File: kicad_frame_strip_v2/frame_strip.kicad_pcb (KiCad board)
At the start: 2 copper layers, 42.5 x 58.5 mm, 61 parts, among them J1 PROGRAM, J10 HEADER_1, J11 HEADER_1, J12 HEADER_1, J2 USART2, J3 HEADER_4, J4 HEADER_4, J5 HEADER_4, J6 HEADER_2, J7 DC_POWER_JACK, J8 SPI1, J9 HEADER_1, Q1 MOS_N_GDS, Q2 MOS_N_GDS, Q3 MOS_N_GDS, Q4 MOS_N_GDS, Q5 MOS_N_GDS, Q6 MOS_N_GDS, Q7 MOS_N_GDS, Q8 MOS_N_GDS, Q9 MOS_N_GDS, SW1 SW_PUSH, SW2 SW_PUSH, SW3 SW_SPDT, U1 STM32F100_LQFP48, U6 sot223

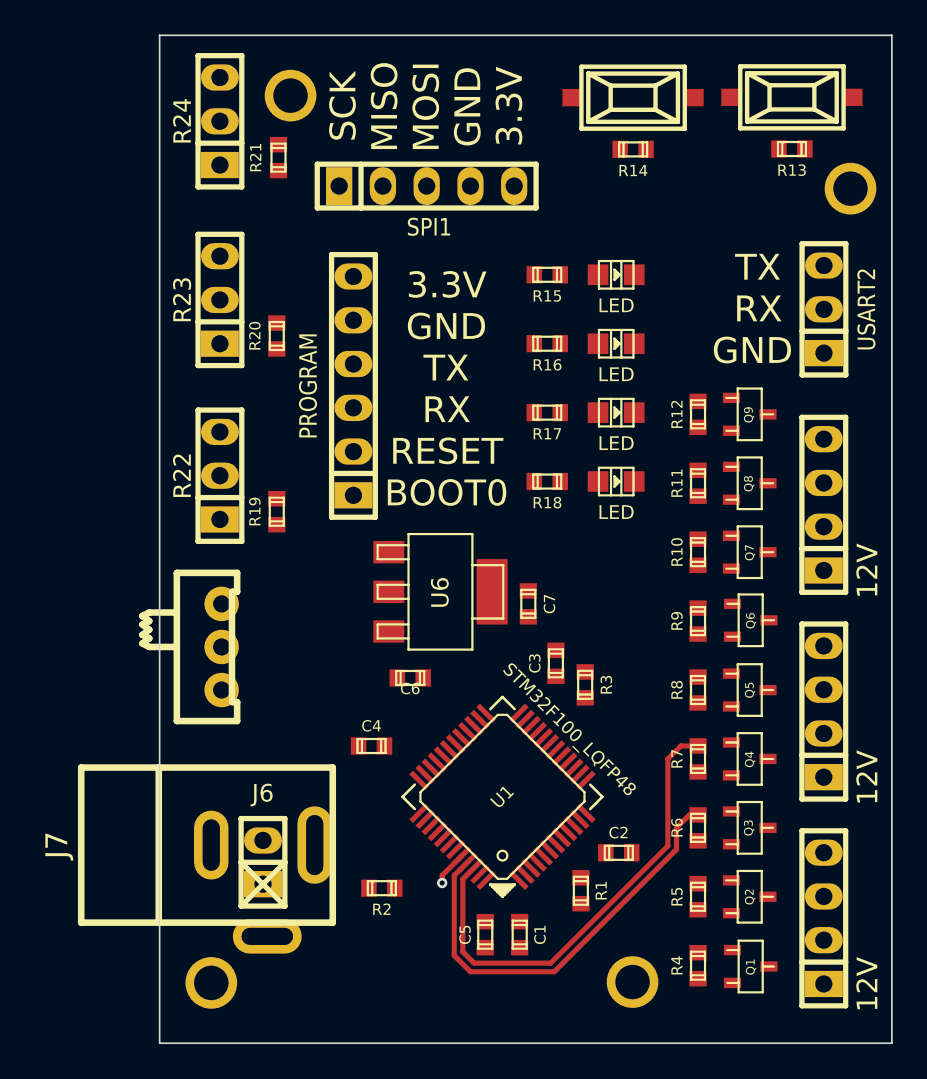
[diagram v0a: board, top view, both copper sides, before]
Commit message: PCB, code
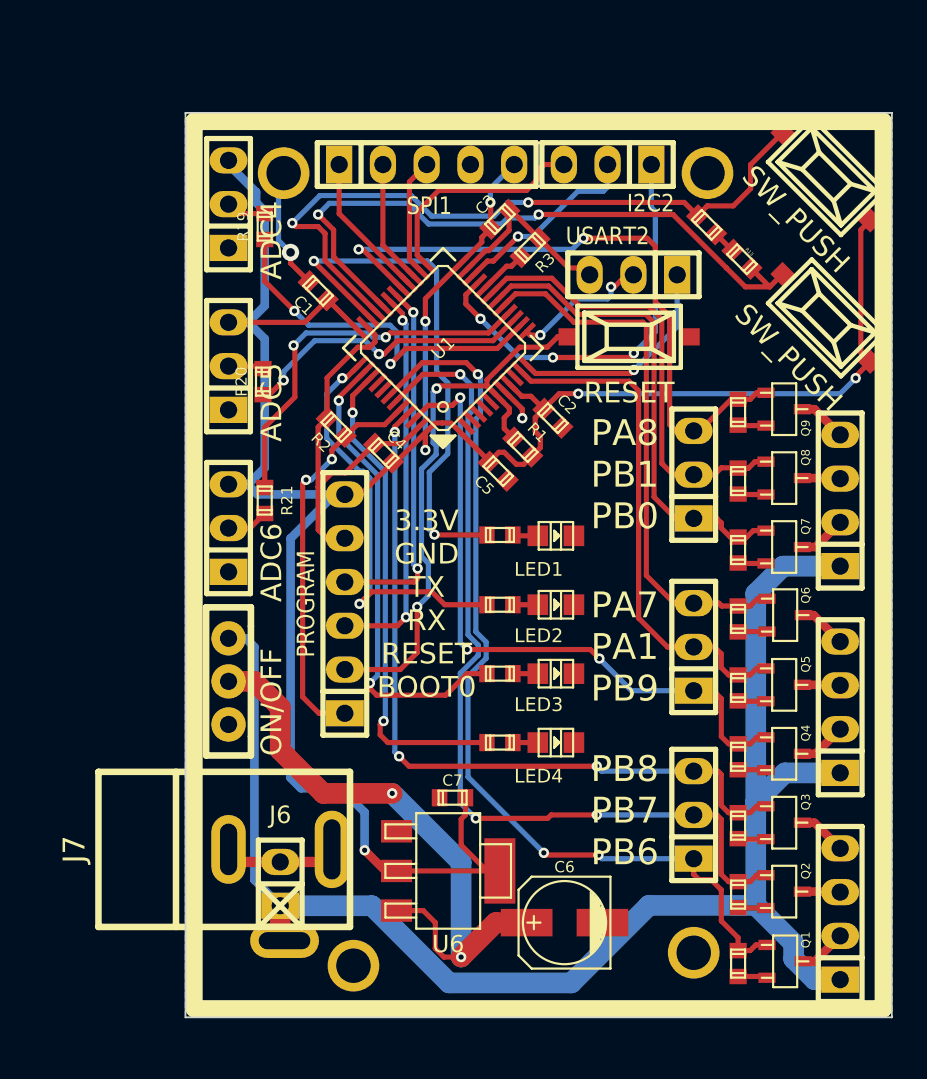
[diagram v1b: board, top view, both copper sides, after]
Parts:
- removed R22, R23: POT, w_pin_strip:pin_socket_3
- added ADC5: POT, w_pin_strip:pin_socket_3, F.Cu at (131.0, 98.2)
- added ADC6: POT, w_pin_strip:pin_socket_3, F.Cu at (131.0, 107.6)
- added J13: HEADER_3, w_pin_strip:pin_socket_3, F.Cu at (158.0, 124.2)
- added J14: HEADER_3, w_pin_strip:pin_socket_3, F.Cu at (158.0, 114.5)
- added J15: HEADER_3, w_pin_strip:pin_socket_3, F.Cu at (158.0, 104.5)
- added J16: I2C2, w_pin_strip:pin_socket_3, F.Cu at (153.0, 86.5)
- added SW4: RESET, w_switch:smd_push, F.Cu at (154.2, 96.5)
- C6: footprint w_smd_cap:c_0603 -> w_smd_cap:c_elec_5x5.3
- LD1: value LED -> LED1
- LD2: value LED -> LED2
- LD3: value LED -> LED3
- LD4: value LED -> LED4
- SW3: value SW_SPDT -> ON/OFF
- moved C1 39.2 mm to (136.2, 93.8), turned to 315 degrees
- moved C5 26.9 mm to (146.7, 104.3), turned to 135 degrees
- moved R2 26.9 mm to (137.2, 101.8), turned to 135 degrees
- moved U1 26.3 mm to (143.4, 97.2)
- moved C3 26.0 mm to (146.8, 89.7), turned to 225 degrees
- moved R1 26.0 mm to (148.1, 102.9), turned to 315 degrees
- moved R3 25.6 mm to (148.5, 91.3), turned to 45 degrees
- moved C2 25.5 mm to (149.8, 101.2), turned to 135 degrees
- moved R21 19.9 mm to (133.1, 106.0), turned to 270 degrees
- moved C4 17.0 mm to (140.0, 103.2), turned to 315 degrees
- moved C6 16.8 mm to (150.5, 130.5)
- moved R19 16.6 mm to (133.1, 90.1)
- moved U6 16.2 mm to (143.8, 127.5)
- moved LD1 15.5 mm to (150.0, 108.0)
- moved LD2 15.5 mm to (150.0, 112.0)
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- renumbered R24 to ADC4
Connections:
- ADC4 pad 2: Net-(R21-Pad1) -> Net-(ADC4-Pad2)
- C6 pad 1: /12V -> Net-(C6-Pad1)
- J7 pad 1: Net-(J7-Pad1) -> /12V
- J8 pad 1: /SPI1_SCK -> /SPI1_MOSI
- J8 pad 3: /SPI1_MOSI -> /SPI1_SCK
- R19 pad 1: Net-(R19-Pad1) -> Net-(ADC4-Pad2)
- R21 pad 1: Net-(R21-Pad1) -> Net-(ADC6-Pad2)
- SW3 pad 1: Net-(J7-Pad1) -> /12V
- SW3 pad 2: /12V -> Net-(C6-Pad1)
- U1 pad 21: /LED2 -> /SCL
- U1 pad 22: /LED3 -> /SDA
- U1 pad 25: /LED4 -> /PB12
- U1 pad 34: (no net) -> /LED1
- U1 pad 37: (no net) -> /LED2
- U1 pad 38: (no net) -> /LED3
- U1 pad 39: (no net) -> /LED4
- U1 pad 41: /LED1 -> (no net)
- U6 pad 3: /12V -> Net-(C6-Pad1)
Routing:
- net +3.3V: track 0.00 -> 147.2 mm, vias 0 -> 6
- net /12V: track 0.00 -> 87.3 mm
- net GND: track 0.00 -> 65.9 mm, vias 0 -> 2
- net /TIM4_CH1: track 0.00 -> 54.1 mm, vias 0 -> 3
- net /TIM4_CH2: track 0.00 -> 52.1 mm, vias 0 -> 3
- net /SW2: track 0.00 -> 41.1 mm, vias 0 -> 2
- net /TIM1_CH1: track 0.00 -> 39.5 mm, vias 0 -> 2
- net /SW1: track 0.00 -> 38.5 mm, vias 0 -> 2
- net Net-(C6-Pad1): track 0.00 -> 35.2 mm, vias 0 -> 2
- net /RESET: track 0.00 -> 34.5 mm, vias 0 -> 2
- net /TIM3_CH2: track 0.00 -> 31.9 mm
- net /LED1: track 0.00 -> 31.4 mm, vias 0 -> 2
- net /TIM2_CH2: track 0.00 -> 29.9 mm
- net /TIM3_CH3: track 0.00 -> 29.4 mm
- net /LED4: track 0.00 -> 28.5 mm, vias 0 -> 2
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- added copper zone on B.Cu, net GND
- added copper zone on F.Cu, net GND
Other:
- board size 42.5 x 58.5 mm -> 41 x 52.5 mm
- net class Default: clearance 0.2 -> 0.15
- rule trace_clearance: 0.2 -> 0.15
- board text added: "B12 SDA SCL"
- board text added: "GND RX TX"
- board text added: "MOSI MISO SCK GND 3.3V"
- board text added: "PA7 PA1 PB9"
- board text added: "PA8 PB1 PB0"
- board text added: "PB8 PB7 PB6"
- board text removed: "SCK MISO MOSI GND 3.3V"
- board text removed: "TX RX GND"

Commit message: Version 3 PCB
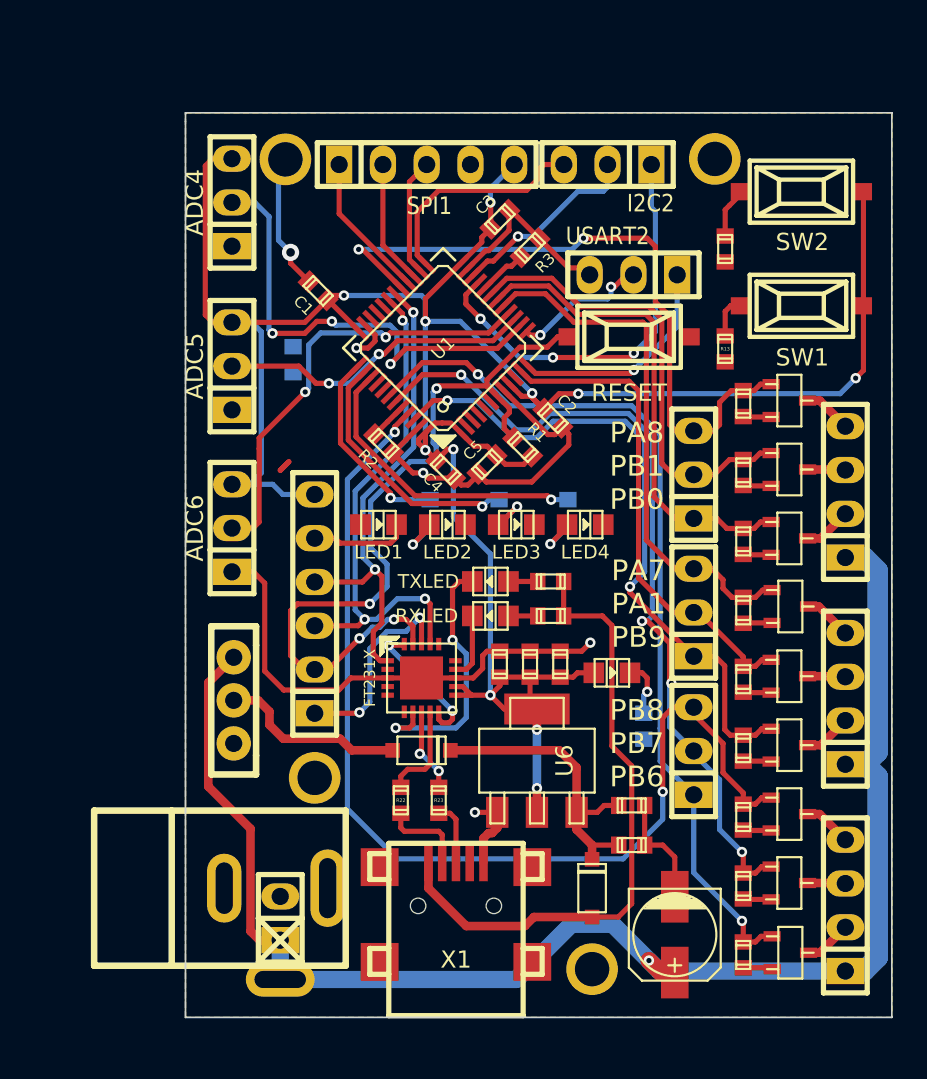
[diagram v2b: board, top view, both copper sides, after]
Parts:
- added C10: C, w_smd_cap:c_0603, F.Cu at (148.5, 115.5)
- added C11: C, w_smd_cap:c_0603, F.Cu at (150.2, 115.5)
- added C8: C, w_smd_cap:c_0603, F.Cu at (154.4, 126.0)
- added C9: C, w_smd_cap:c_0603, F.Cu at (154.4, 123.7)
- added D1: SCHOTTKY, w_smd_diode:sod123, F.Cu at (152.1, 128.5)
- added D2: SCHOTTKY, w_smd_diode:sod123, F.Cu at (142.2, 120.5)
- added LD5: RXLED, w_smd_leds:Led_0805, F.Cu at (146.2, 112.7)
- added LD6: TXLED, w_smd_leds:Led_0805, F.Cu at (146.2, 110.7)
- added LD7: ON, w_smd_leds:Led_0805, F.Cu at (153.2, 116.0)
- added R22: R, w_smd_resistors:r_0603, F.Cu at (141.0, 123.4)
- added R23: R, w_smd_resistors:r_0603, F.Cu at (143.2, 123.4)
- added U2: FT231X, w_smd_qfn:qfn-20, F.Cu at (142.2, 116.3)
- added X1: MINI-USB_SHIELD5P2-32005-601, w_conn_pc:conn_usb_B_mini_smd, F.Cu at (144.2, 130.9)
- R15, R16, R17, R18, R21: moved to B.Cu
- SW1: value SW_PUSH -> SW1
- SW2: value SW_PUSH -> SW2
- moved R19 28.0 mm to (149.7, 112.7), turned to 0 degrees
- moved R21 25.6 mm to (155.1, 119.1)
- moved R20 20.3 mm to (149.7, 110.7), turned to 180 degrees
- moved R15 15.7 mm to (134.8, 97.8), turned to 90 degrees
- moved R18 13.9 mm to (150.7, 106.7), turned to 90 degrees
- moved LD4 12.8 mm to (151.7, 107.4)
- moved J10 11.1 mm to (136.0, 122.1)
- moved LD1 10.3 mm to (139.7, 107.4)
- moved R17 9.35 mm to (146.7, 106.7), turned to 90 degrees
- moved LD3 8.95 mm to (147.7, 107.4)
- moved C7 8.22 mm to (146.8, 115.5), turned to 270 degrees
- moved U6 8.21 mm to (148.9, 121.1), turned to 0 degrees
- moved LD2 7.83 mm to (143.7, 107.4)
- moved R16 6.71 mm to (142.7, 106.7), turned to 90 degrees
- moved C6 6.44 mm to (156.9, 131.2), turned to 270 degrees
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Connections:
- ADC4 pad 2: Net-(ADC4-Pad2) -> /ADC1_4
- ADC5 pad 2: Net-(ADC5-Pad2) -> /ADC1_5
- ADC6 pad 2: Net-(ADC6-Pad2) -> /ADC1_6
- C6 pad 1: Net-(C6-Pad1) -> /12V
- R19 pad 1: Net-(ADC4-Pad2) -> /V_USB
- R19 pad 2: /ADC1_4 -> Net-(LD5-Pad1)
- R20 pad 1: Net-(ADC5-Pad2) -> Net-(LD6-Pad1)
- R20 pad 2: /ADC1_5 -> /V_USB
- R21 pad 1: Net-(ADC6-Pad2) -> GND
- R21 pad 2: /ADC1_6 -> Net-(LD7-Pad2)
- SW3 pad 2: Net-(C6-Pad1) -> Net-(D2-Pad1)
- U6 pad 3: Net-(C6-Pad1) -> Net-(C8-Pad1)
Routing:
- net /SW2: track 41.1 -> 2.92 mm, vias 2 -> 0
- net GND: track 65.9 -> 102.4 mm, vias 2 -> 5
- net /V_USB: track 0.00 -> 36.4 mm
- net /SW1: track 38.5 -> 2.88 mm, vias 2 -> 0
- net Net-(C6-Pad1): track 35.2 -> 0.00 mm, vias 2 -> 0
- net /LED1: track 31.4 -> 0.00 mm, vias 2 -> 0
- net Net-(C8-Pad1): track 0.00 -> 17.6 mm
- net /TIM4_CH3: track 44.2 -> 61.4 mm, vias 3 -> 2
- net Net-(LD6-Pad2): track 0.00 -> 15.3 mm, vias 0 -> 2
- net /LED3: track 27.7 -> 15.0 mm, vias 2 -> 1
- net /LED2: track 24.2 -> 11.8 mm, vias 2 -> 1
- net /RESET: track 34.5 -> 46.6 mm, vias 2 -> 4
- net Net-(D2-Pad1): track 0.00 -> 10.9 mm
- net /LED4: track 28.5 -> 17.7 mm, vias 2 -> 1
- net /BOOT0: track 23.2 -> 14.1 mm
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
